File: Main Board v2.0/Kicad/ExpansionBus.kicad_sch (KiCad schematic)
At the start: 11 parts, among them J1 Bus_ISA_16bit, U13 74HC245, U14 74HC245, U15 74HC245, U17 74HC646, U18 74HC646

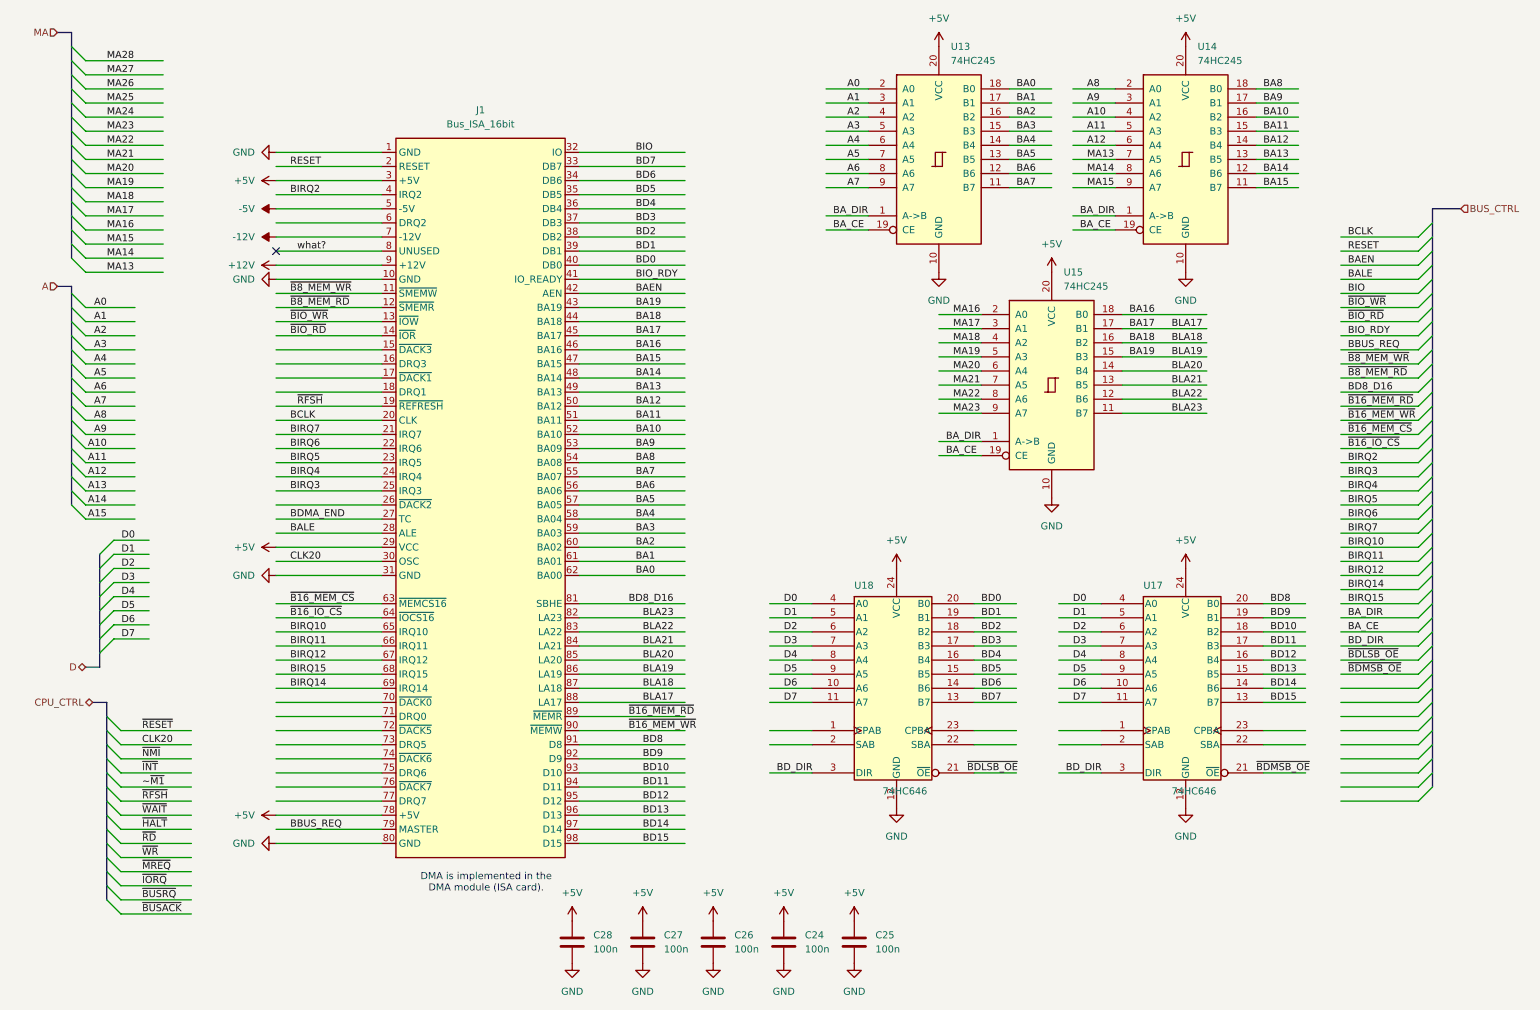
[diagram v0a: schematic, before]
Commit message: schematic done*
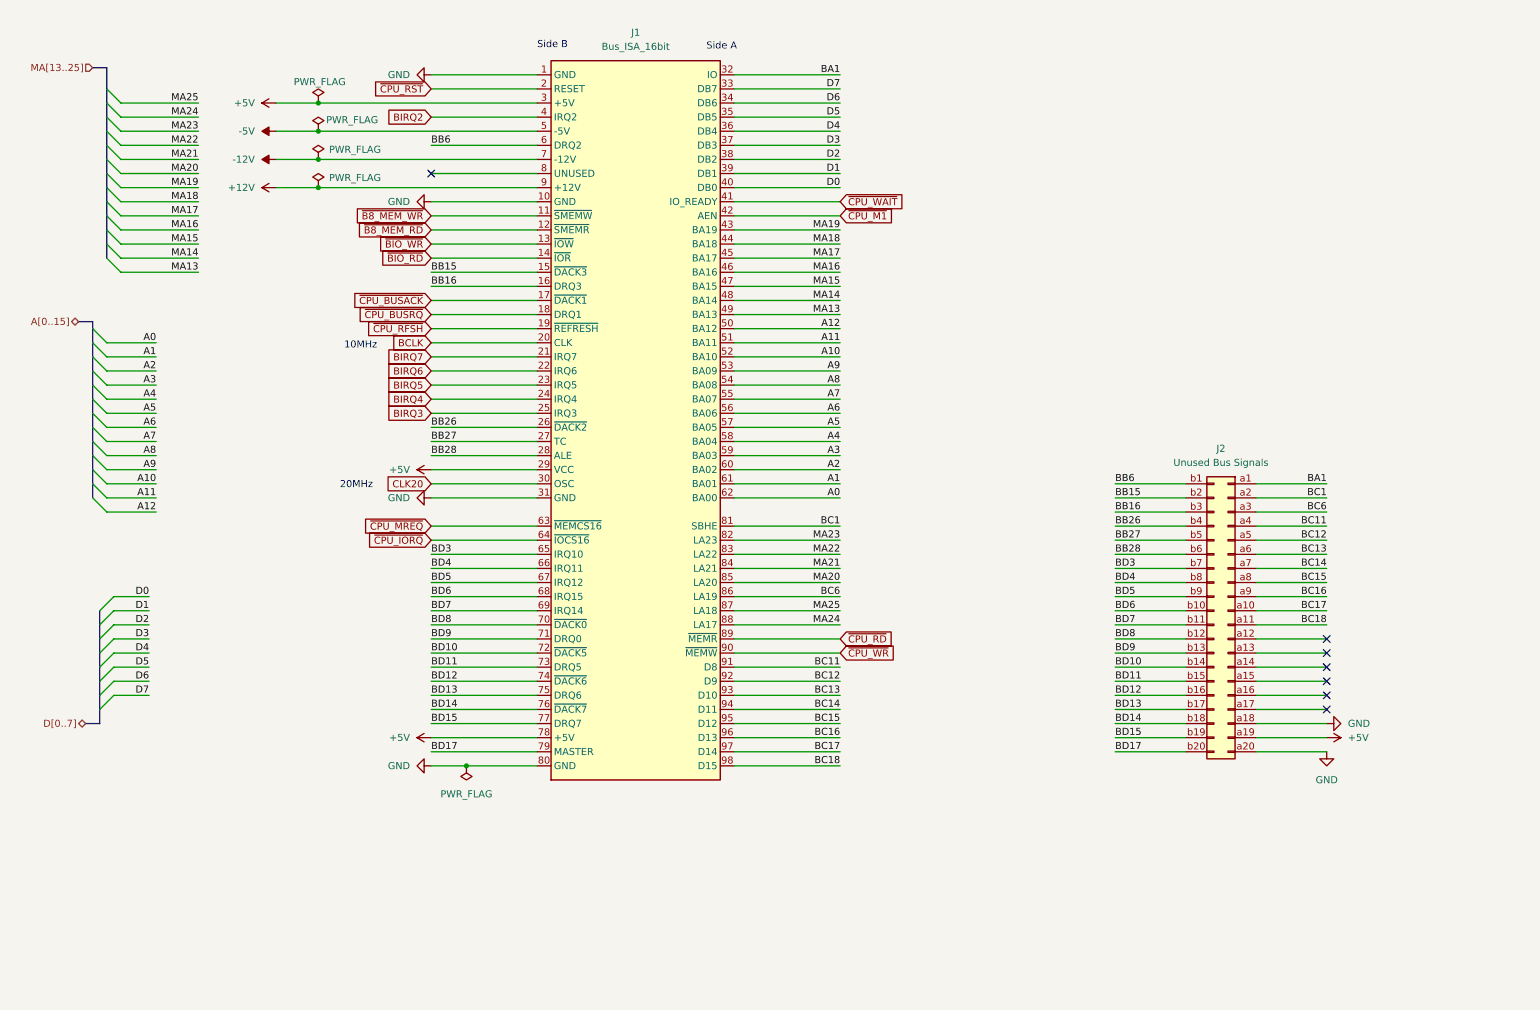
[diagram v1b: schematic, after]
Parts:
- removed C24, C25, C26, C27, C28: 100n, symbol Device:C
- removed U13, U14, U15: 74HC245, symbol 74xx:74HC245
- removed U17, U18: 74HC646, symbol My-74-Logic:74HC646
- added J2: Unused Bus Signals, Connector_PinSocket_2.54mm:PinSocket_2x20_P2.54mm_Vertical, symbol Connector_Generic:Conn_02x20_Row_Letter_First
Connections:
- net BA0 is gone; now on net A0: J1.62 (BA00)
- net BA10 is gone; now on net A10: J1.52 (BA10)
- net BA11 is gone; now on net A11: J1.51 (BA11)
- net BA12 is gone; now on net A12: J1.50 (BA12)
- net BA13 is gone; now on net MA13: J1.49 (BA13)
- net BA14 is gone; now on net MA14: J1.48 (BA14)
- net BA15 is gone; now on net MA15: J1.47 (BA15)
- net BA16 is gone; now on net MA16: J1.46 (BA16)
- net BA2 is gone; now on net A2: J1.60 (BA02)
- net BA3 is gone; now on net A3: J1.59 (BA03)
- net BA4 is gone; now on net A4: J1.58 (BA04)
- net BA5 is gone; now on net A5: J1.57 (BA05)
- net BA6 is gone; now on net A6: J1.56 (BA06)
- net BA7 is gone; now on net A7: J1.55 (BA07)
- net BA8 is gone; now on net A8: J1.54 (BA08)
- net BA9 is gone; now on net A9: J1.53 (BA09)
- net BD0 is gone; now on net D0: J1.40 (DB0)
- net BD1 is gone; now on net D1: J1.39 (DB1)
- net BD2 is gone; now on net D2: J1.38 (DB2)
- net BIO is gone; now on net BA1: J1.32 (IO)
- net BIRQ10 is gone; now on net BD3: J1.65 (IRQ10)
- net BIRQ11 is gone; now on net BD4: J1.66 (IRQ11)
- net BIRQ12 is gone; now on net BD5: J1.67 (IRQ12)
- net BIRQ14 is gone; now on net BD7: J1.69 (IRQ14)
- net BIRQ15 is gone; now on net BD6: J1.68 (IRQ15)
- net BLA20 is gone; now on net MA20: J1.85 (LA20)
- net BLA21 is gone; now on net MA21: J1.84 (LA21)
- net BLA22 is gone; now on net MA22: J1.83 (LA22)
- net BLA23 is gone; now on net MA23: J1.82 (LA23)
- net +5V: now also J2.a19 (Pin_a19)
- net A1: now also J1.61 (BA01)
- net BA1: now also J2.a1 (Pin_a1); no longer J1.61 (BA01)
- net BD10: now also J1.72 (~{DACK5}), J2.b14 (Pin_b14); no longer J1.93 (D10)
- net BD11: now also J1.73 (DRQ5), J2.b15 (Pin_b15); no longer J1.94 (D11)
- net BD12: now also J1.74 (~{DACK6}), J2.b16 (Pin_b16); no longer J1.95 (D12)
- net BD13: now also J1.75 (DRQ6), J2.b17 (Pin_b17); no longer J1.96 (D13)
- net BD14: now also J1.76 (~{DACK7}), J2.b18 (Pin_b18); no longer J1.97 (D14)
- net BD15: now also J1.77 (DRQ7), J2.b19 (Pin_b19); no longer J1.98 (D15)
- net BD3: now also J2.b7 (Pin_b7); no longer J1.37 (DB3)
- net BD4: now also J2.b8 (Pin_b8); no longer J1.36 (DB4)
- net BD5: now also J2.b9 (Pin_b9); no longer J1.35 (DB5)
- net BD6: now also J2.b10 (Pin_b10); no longer J1.34 (DB6)
- net BD7: now also J2.b11 (Pin_b11); no longer J1.33 (DB7)
- net BD8: now also J1.70 (~{DACK0}), J2.b12 (Pin_b12); no longer J1.91 (D8)
- net BD9: now also J1.71 (DRQ0), J2.b13 (Pin_b13); no longer J1.92 (D9)
- net D3: now also J1.37 (DB3)
- net D4: now also J1.36 (DB4)
- net D5: now also J1.35 (DB5)
- net D6: now also J1.34 (DB6)
- net D7: now also J1.33 (DB7)
- net GND: now also J2.a18 (Pin_a18), J2.a20 (Pin_a20)
- net MA17: now also J1.45 (BA17)
- net MA18: now also J1.44 (BA18)
- net MA19: now also J1.43 (BA19)
- net MA24: now also J1.88 (LA17)
- net MA25: now also J1.87 (LA18)
- net BB15: now reaches J1.15 (~{DACK3})
- net BB15: now also J2.b2 (Pin_b2)
- net BB16: now reaches J1.16 (DRQ3)
- net BB16: now also J2.b3 (Pin_b3)
- net ~{CPU_BUSACK}: now reaches J1.17 (~{DACK1})
- net ~{CPU_BUSRQ}: now reaches J1.18 (DRQ1)
- net BB26: now reaches J1.26 (~{DACK2})
- net BB26: now also J2.b4 (Pin_b4)
- net BB6: now reaches J1.6 (DRQ2)
- net BB6: now also J2.b1 (Pin_b1)
- removed net BA17: J1.45 (BA17), J1.88 (LA17)
- removed net BA18: J1.44 (BA18), J1.87 (LA18)
- net BA19 renamed BC6
- net BC6: now also J2.a3 (Pin_a3); no longer J1.43 (BA19)
- net BAEN renamed ~{CPU_M1}
- net BALE renamed BB28
- net BB28: now also J2.b6 (Pin_b6)
- net BBUS_REQ renamed BD17
- net BD17: now also J2.b20 (Pin_b20)
- net BD8_D16 renamed BC1
- net BC1: now also J2.a2 (Pin_a2)
- net BDMA_END renamed BB27
- net BB27: now also J2.b5 (Pin_b5)
- net BIO_RDY renamed ~{CPU_WAIT}
- net RESET renamed ~{CPU_RST}
- net what?: no longer names the net of J1.8 (UNUSED)
- net ~{B16_IO_CS} renamed ~{CPU_IORQ}
- net ~{B16_MEM_CS} renamed ~{CPU_MREQ}
- net ~{B16_MEM_RD} renamed ~{CPU_RD}
- net ~{B16_MEM_WR} renamed ~{CPU_WR}
- net ~{RFSH} renamed ~{CPU_RFSH}
- new net BC11: J1.91 (D8), J2.a4 (Pin_a4)
- new net BC12: J1.92 (D9), J2.a5 (Pin_a5)
- new net BC13: J1.93 (D10), J2.a6 (Pin_a6)
- new net BC14: J1.94 (D11), J2.a7 (Pin_a7)
- new net BC15: J1.95 (D12), J2.a8 (Pin_a8)
- new net BC16: J1.96 (D13), J2.a9 (Pin_a9)
- new net BC17: J1.97 (D14), J2.a10 (Pin_a10)
- new net BC18: J1.98 (D15), J2.a11 (Pin_a11)
- no-connect marks 1 -> 7
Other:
- note added: "10MHz"
- note added: "20MHz"
- note added: "Side A"
- note added: "Side B"
- note removed: "DMA is implemented in the DMA module (ISA card)."
- moved on the sheet: J1
